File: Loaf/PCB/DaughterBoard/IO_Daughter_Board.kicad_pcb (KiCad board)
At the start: 2 copper layers, 93 x 55.7 mm, 12 parts, among them J1 I/O Block, J2 5V Block, J3 DB25_Socket, J4 Ground Block, J5 Ground Block, J6 Barrel Jack, SW1 ESTOP, SW2 RESET

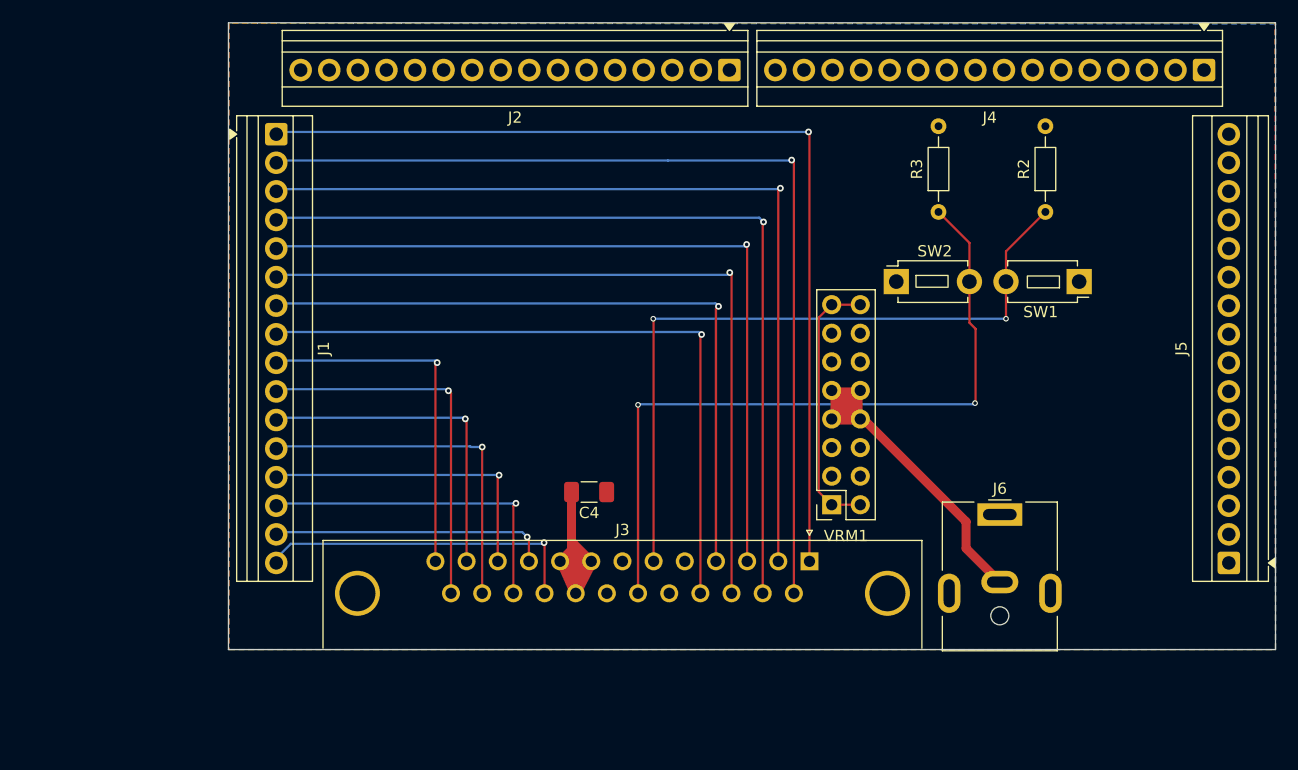
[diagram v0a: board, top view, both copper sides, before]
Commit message: Updated Daughter Board
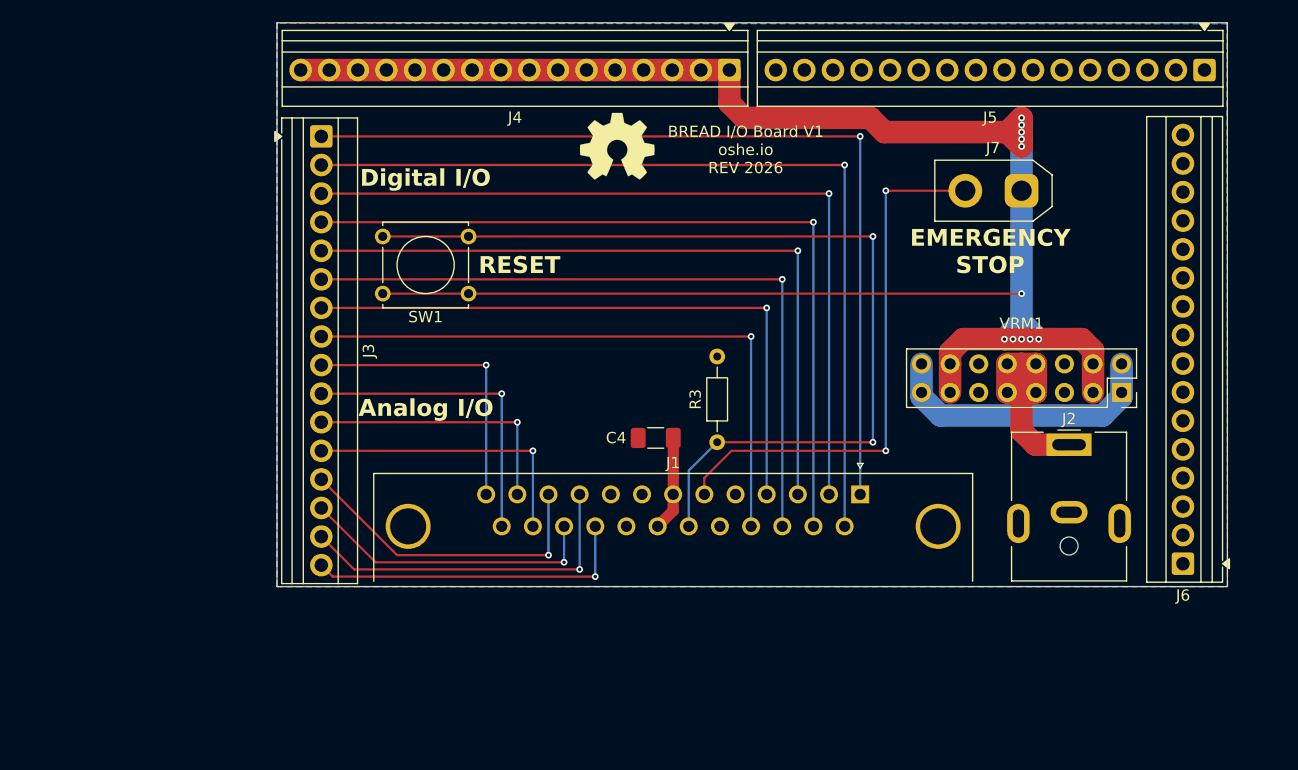
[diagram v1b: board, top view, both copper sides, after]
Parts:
- removed R2: 10K, Resistor_THT:R_Axial_DIN0204_L3.6mm_D1.6mm_P7.62mm_Horizontal
- removed SW2: RESET, Button_Switch_THT:SW_PUSH_1P1T_6x3.5mm_H5.0_APEM_MJTP1250
- added J7: Screw_Terminal_01x02, Connector_AMASS:AMASS_XT30UPB-M_1x02_P5.0mm_Vertical, F.Cu at (170.4, 77.7)
- added Logo1: Logo_Open_Hardware_Small, Symbol:OSHW-Symbol_6.7x6mm_SilkScreen, F.Cu at (134.5, 73.8)
- SW1: value ESTOP -> SW_Push; footprint Button_Switch_THT:SW_PUSH_1P1T_6x3.5mm_H5.0_APEM_MJTP1250 -> Button_Switch_THT:SW_Tactile_Straight_KSL0Axx1LFTR
- moved SW1 54.3 mm to (121.3, 86.9)
- moved R3 28.4 mm to (143.4, 100.1)
- moved VRM1 27.6 mm to (179.3, 95.7), turned to -90 degrees
- moved J2 8.74 mm to (174.7, 100.3)
- moved C4 7.63 mm to (137.9, 99.7)
- moved J1 7.47 mm to (156.1, 104.7)
- moved J6 4.08 mm to (184.8, 110.9)
- moved J3 4.01 mm to (108.2, 72.9)
- renumbered J3 to J1, J6 to J2, J1 to J3, J2 to J4, J4 to J5, J5 to J6
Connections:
- C4 pad 1: +5V -> +5V Slice
- J1 pad 20: +5V -> +5V Slice
- J1 pad 7: +5V -> +5V Slice
- J2 pad 1: GND -> +12V
- J2 pad 2: +12V -> GND
- SW1 pad 2: /ESTOP -> /RESET
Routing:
- net +5V: track 0.00 -> 178.9 mm, vias 0 -> 11
- net /RESET: track 65.1 -> 84.2 mm
- net /ESTOP: track 63.9 -> 48.8 mm
- net GND: track 13.5 -> 0.00 mm
- net +5V Slice: track 0.00 -> 8.43 mm
- net /DIO2: track 78.3 -> 71.9 mm
- net /DIO4: track 70.2 -> 64.0 mm
- net /DIO5: track 69.1 -> 62.9 mm
- net /DIO6: track 62.4 -> 56.2 mm
- net /AIO0: track 32.3 -> 26.1 mm
- net /DIO7: track 61.1 -> 55.1 mm
- net /AIO3: track 31.5 -> 25.5 mm
- net /DIO0: track 85.7 -> 79.7 mm
- net /DIO1: track 84.6 -> 78.6 mm
- net /AIO6: track 24.9 -> 30.8 mm
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- added copper zone on F.Cu, net GND
- removed copper zone on F.Cu, net +5V
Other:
- board size 93 x 55.7 mm -> 84.5 x 50.1 mm
- board text added: "Analog I/O"
- board text added: "BREAD I/O Board V1 oshe.io REV 2026"
- board text added: "Digital I/O"
- board text added: "EMERGENCY STOP"
- board text added: "RESET"

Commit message: See Description
Rebuilt I/O Slice daughter board.
Added transmission to the Input slice.
Got digital reading working on input slice.
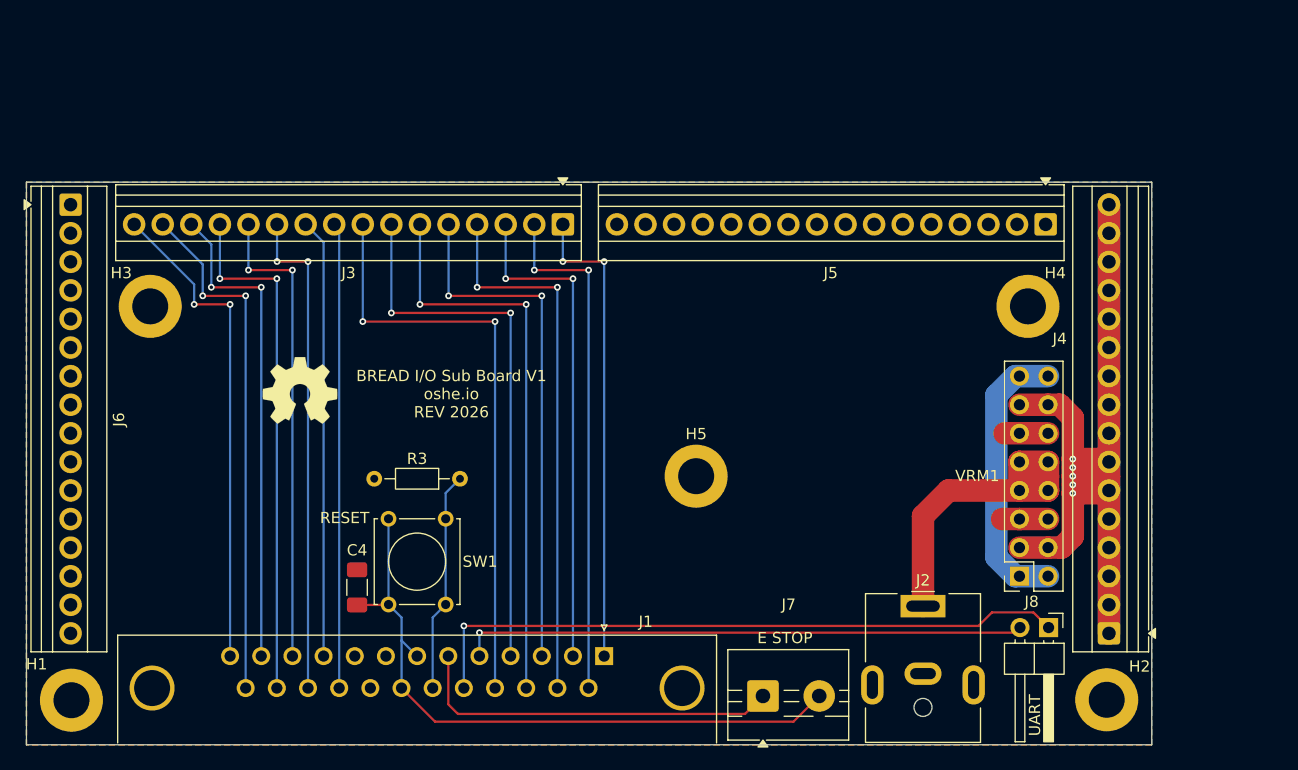
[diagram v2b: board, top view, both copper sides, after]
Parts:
- added H1: MountingHole_Pad, MountingHole:MountingHole_3.2mm_M3_DIN965_Pad, F.Cu at (86.0, 123.0)
- added H2: MountingHole_Pad, MountingHole:MountingHole_3.2mm_M3_DIN965_Pad, F.Cu at (178.0, 123.0)
- added H3: MountingHole_Pad, MountingHole:MountingHole_3.2mm_M3_DIN965_Pad, F.Cu at (93.0, 88.0)
- added H4: MountingHole_Pad, MountingHole:MountingHole_3.2mm_M3_DIN965_Pad, F.Cu at (171.0, 88.0)
- added H5: MountingHole_Pad, MountingHole:MountingHole_3.2mm_M3_DIN965_Pad, F.Cu at (141.5, 103.1)
- added J8: Conn_01x02_Pin, Connector_PinHeader_2.54mm:PinHeader_1x02_P2.54mm_Horizontal, F.Cu at (172.8, 116.5)
- J7: footprint Connector_AMASS:AMASS_XT30UPB-M_1x02_P5.0mm_Vertical -> TerminalBlock:TerminalBlock_MaiXu_MX126-5.0-02P_1x02_P5.00mm
- moved J6 103.9 mm to (85.9, 79.0), turned to -90 degrees
- moved J4 60.4 mm to (178.2, 117.1), turned to 90 degrees
- moved J7 50.4 mm to (147.4, 122.6), turned to 0 degrees
- moved Logo1 35.6 mm to (106.3, 95.5)
- moved C4 29.7 mm to (111.4, 113.0), turned to 90 degrees
- moved SW1 28.5 mm to (114.2, 114.5), turned to 90 degrees
- moved J1 26.9 mm to (133.3, 119.1)
- moved R3 23.1 mm to (120.5, 103.3), turned to 180 degrees
- moved J3 22.8 mm to (129.7, 80.7), turned to 180 degrees
- moved J5 19.7 mm to (172.6, 80.7)
- moved J2 19.3 mm to (161.7, 114.6)
- moved VRM1 18.7 mm to (170.2, 112.0), turned to 180 degrees
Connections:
- J3 pad 10: /AIO1 -> /AIO6
- J3 pad 11: /AIO2 -> /AIO5
- J3 pad 12: /AIO3 -> /AIO4
- J3 pad 13: /AIO4 -> /AIO3
- J3 pad 14: /AIO5 -> /AIO2
- J3 pad 15: /AIO6 -> /AIO1
- J3 pad 16: /AIO7 -> /AIO0
- J3 pad 9: /AIO0 -> /AIO7
- J7 pad 1: +5V -> /ESTOP
- J7 pad 2: /ESTOP -> +5V Slice
- SW1 pad 1: +5V -> +5V Slice
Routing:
- net /RESET: track 84.2 -> 19.6 mm, vias 2 -> 0
- net +5V: track 178.9 -> 114.4 mm, vias 11 -> 5
- net /URX: track 0.00 -> 58.5 mm, vias 0 -> 1
- net +5V Slice: track 8.43 -> 59.6 mm
- net /UTX: track 0.00 -> 50.3 mm, vias 0 -> 1
- net /DIO0: track 79.7 -> 42.0 mm, vias 1 -> 2
- net /DIO1: track 78.6 -> 46.0 mm, vias 1 -> 2
- net /DIO2: track 71.9 -> 44.3 mm, vias 1 -> 2
- net /DIO3: track 70.8 -> 48.6 mm, vias 1 -> 2
- net /AIO3: track 25.5 -> 46.3 mm, vias 1 -> 2
- net /AIO2: track 23.8 -> 43.5 mm, vias 1 -> 2
- net /AIO1: track 27.8 -> 46.5 mm, vias 1 -> 2
- net /AIO0: track 26.1 -> 43.8 mm, vias 1 -> 2
- net /DIO4: track 64.0 -> 46.7 mm, vias 1 -> 2
- net /AIO5: track 26.8 -> 44.0 mm, vias 1 -> 2
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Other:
- board size 84.5 x 50.1 mm -> 100 x 50 mm
- board text added: "BREAD I/O Sub Board V1 oshe.io REV 2026"
- board text added: "E STOP"
- board text added: "UART"
- board text removed: "Analog I/O"
- board text removed: "BREAD I/O Board V1 oshe.io REV 2026"
- board text removed: "Digital I/O"
- board text removed: "EMERGENCY STOP"
